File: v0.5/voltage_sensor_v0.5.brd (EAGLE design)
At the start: 73 x 118 mm, 64 parts, among them IC1 AP2112K-3.3TRG1, J1 1017505, J2 20020316-H021B01LF, J9 RJ11-6, M1 MOV-14D431KTR, M2 MOV-14D431KTR, M3 MOV-14D431KTR, T1 ZMPT101B, T2 ZMPT101B, T3 ZMPT101B

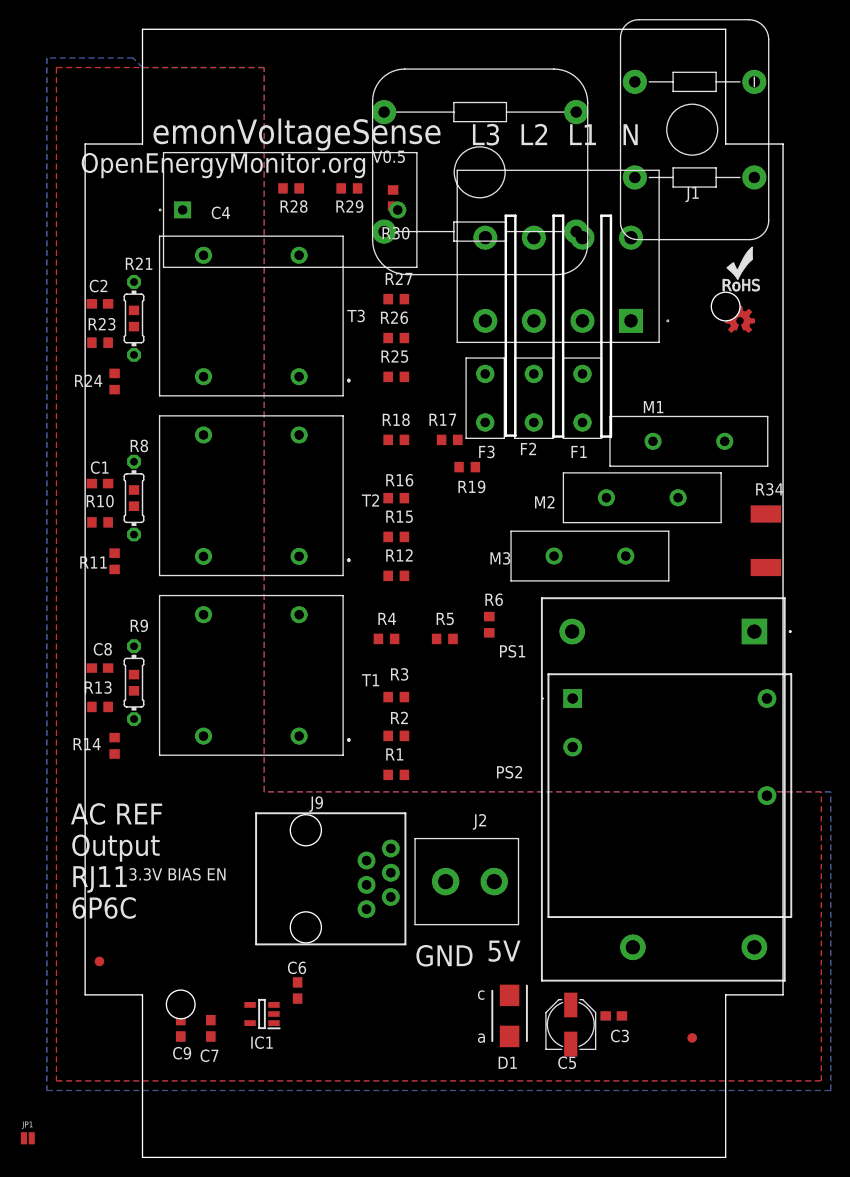
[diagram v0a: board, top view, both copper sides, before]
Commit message: new design
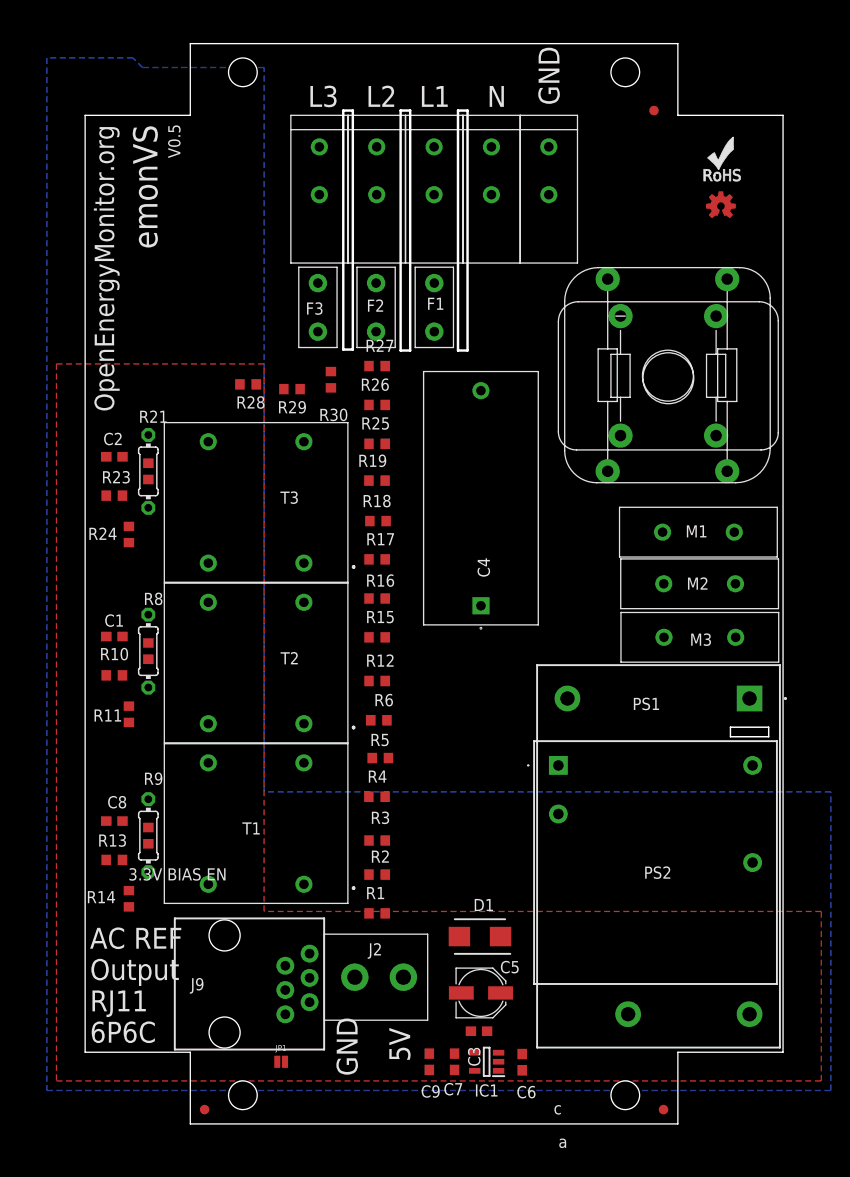
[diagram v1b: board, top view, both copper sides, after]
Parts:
- removed J1: 1017505, 1017505:1017505
- removed R34: 12R 3W, rcl:R2512
- added U$3, U$5, U$6, U$7, U$8: 1905010, Phoenix-Contact-1905010:1905010
- moved C4 51.8 mm to (41.4, 57.7), turned to 90 degrees
- moved U$1 28.6 mm to (61.5, 82.0), turned to 90 degrees
- moved JP1 27.7 mm to (20.5, 10.0)
- moved U$2 27.5 mm to (72.5, 74.0), turned to 90 degrees
- moved C9 26.2 mm to (36.0, 10.0)
- moved C7 25.7 mm to (38.6, 10.0)
- moved C6 24.7 mm to (45.7, 9.96)
- moved IC1 24.0 mm to (42.0, 10.0)
- moved R29 21.8 mm to (21.6, 80.4)
- moved R28 21.0 mm to (17.0, 80.9)
- moved R30 20.1 mm to (25.7, 81.3)
- moved F3 19.9 mm to (26.3, 93.1)
- moved T3 19.5 mm to (22.9, 62.2)
- moved F2 19.0 mm to (32.4, 93.1)
- moved FD1 19.0 mm to (12.5, 5.00)
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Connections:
- net GND: now also U$7.P$1, U$7.P$2
- net L1: now also PS1.1, PS2.2, U$1.P$3, U$2.P$3; no longer F1.OUT, R34.1
- net N$16: now also U$8.P$1, U$8.P$2; no longer J1.7, J1.8
- net N$17: now also C4.2, F1.OUT, U$1.P$4, U$2.P$4; no longer PS1.1, PS2.2, R34.2
- net N$7: now also U$5.P$1, U$5.P$2; no longer J1.3, J1.4
- net N$8: now also U$3.P$1, U$3.P$2; no longer J1.5, J1.6
- net NEUTRAL: now also C4.1, U$1.P$1, U$1.P$2, U$2.P$1, U$2.P$2, U$6.P$1, U$6.P$2; no longer J1.1, J1.2
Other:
- board size 73 x 118 mm -> 73 x 113 mm
- board text added: "emonVS"
- board text removed: "emonVoltageSense"
